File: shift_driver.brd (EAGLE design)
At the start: 100 x 90 mm, 28 parts, among them IC1 7805T, IC2 74HC595D, IC3 74HC595D, IC4 74HC595D, IC5 74HC595D, IC6 74HC595D, IC7 74HC595D

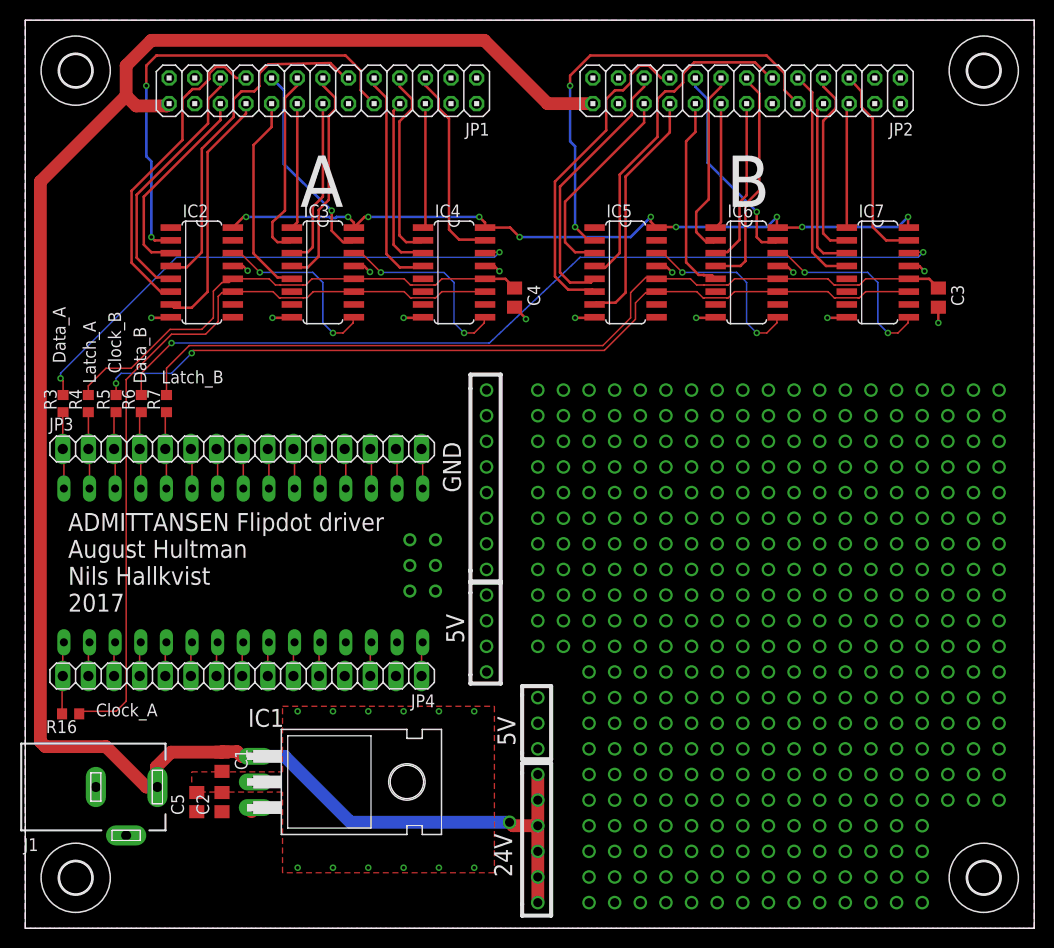
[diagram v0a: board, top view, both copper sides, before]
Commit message: Add code and latest board file
Code for arduino and PC
Minor changes to board file
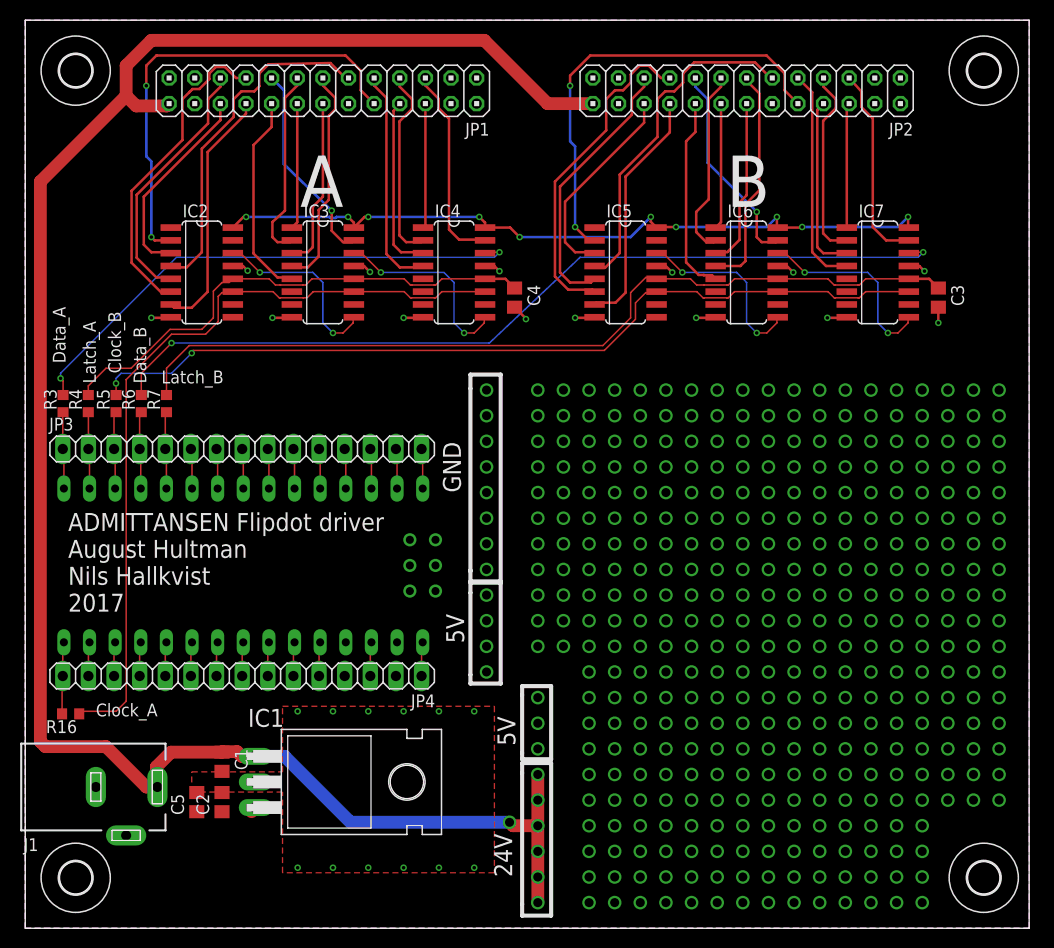
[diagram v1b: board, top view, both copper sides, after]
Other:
- board size 100 x 90 mm -> 99.5 x 90 mm
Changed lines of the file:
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@@
 <?xml version="1.0" encoding="utf-8"?>
 <!DOCTYPE eagle SYSTEM "eagle.dtd">
-<eagle version="8.3.2">
+<eagle version="8.4.2">
 <drawing>
 <settings>
@@
 <layer number="59" name="tCarbon" color="7" fill="1" visible="no" active="no"/>
 <layer number="60" name="bCarbon" color="7" fill="1" visible="no" active="no"/>
-<layer number="88" name="SimResults" color="9" fill="1" visible="no" active="yes"/>
-<layer number="89" name="SimProbes" color="9" fill="1" visible="no" active="yes"/>
+<layer number="88" name="SimResults" color="9" fill="1" visible="no" active="no"/>
+<layer number="89" name="SimProbes" color="9" fill="1" visible="no" active="no"/>
 <layer number="90" name="Modules" color="5" fill="1" visible="no" active="no"/>
 <layer number="91" name="Nets" color="2" fill="1" visible="no" active="no"/>
@@
 <board>
 <plain>
-<wire x1="0" y1="0" x2="100" y2="0" width="0" layer="20"/>
-<wire x1="100" y1="0" x2="100" y2="90" width="0" layer="20"/>
-<wire x1="100" y1="90" x2="0" y2="90" width="0" layer="20"/>
+<wire x1="0" y1="0" x2="99.5" y2="0" width="0" layer="20"/>
+<wire x1="99.5" y1="0" x2="99.5" y2="90" width="0" layer="20"/>
+<wire x1="99.5" y1="90" x2="0" y2="90" width="0" layer="20"/>
 <wire x1="0" y1="90" x2="0" y2="0" width="0" layer="20"/>
 <text x="27.25" y="71.5" size="5.08" layer="21">A</text>
 <text x="69.5" y="71.5" size="5.08" layer="21">B</text>
 <polygon width="0.254" layer="41">
-<vertex x="100" y="55"/>
+<vertex x="99.5" y="55"/>
 <vertex x="44" y="55"/>
 <vertex x="44" y="34.5"/>
@@
 <vertex x="48.5" y="16"/>
 <vertex x="48.5" y="0"/>
-<vertex x="100" y="0"/>
+<vertex x="99.5" y="0"/>
 </polygon>
 <polygon width="0.254" layer="42">
 <vertex x="47" y="55"/>
-<vertex x="100" y="55"/>
-<vertex x="100" y="0"/>
+<vertex x="99.5" y="55"/>
+<vertex x="99.5" y="0"/>
 <vertex x="47.25" y="0"/>
 <vertex x="47.25" y="24"/>
@@
 <param name="dpMaxLengthDifference" value="10mm"/>
 <param name="dpGapFactor" value="2.5"/>
-<param name="checkGrid" value="0"/>
 <param name="checkAngle" value="0"/>
 <param name="checkFont" value="1"/>
 <param name="checkRestrict" value="0"/>
+<param name="checkStop" value="0"/>
 <param name="useDiameter" value="13"/>
 <param name="maxErrors" value="50"/>
@@
 <vertex x="0" y="90"/>
 <vertex x="0" y="0"/>
-<vertex x="100" y="0"/>
-<vertex x="100" y="90"/>
+<vertex x="99.5" y="0"/>
+<vertex x="99.5" y="90"/>
 </polygon>
 <contactref element="C3" pad="2"/>
@@
 <vertex x="0" y="0"/>
 <vertex x="0" y="90"/>
-<vertex x="100" y="90"/>
-<vertex x="100" y="0"/>
+<vertex x="99.5" y="90"/>
+<vertex x="99.5" y="0"/>
 </polygon>
 <via x="27" y="21.5" extent="1-16" drill="0.35"/>
@@
 <polygon width="0.1524" layer="1" isolate="0.3" rank="3">
 <vertex x="0" y="90"/>
-<vertex x="100" y="90"/>
-<vertex x="100" y="0"/>
+<vertex x="99.5" y="90"/>
+<vertex x="99.5" y="0"/>
 <vertex x="0" y="0"/>
 </polygon>
